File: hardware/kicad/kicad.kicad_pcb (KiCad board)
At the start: 2 copper layers, 4 parts, among them U1 RP2040

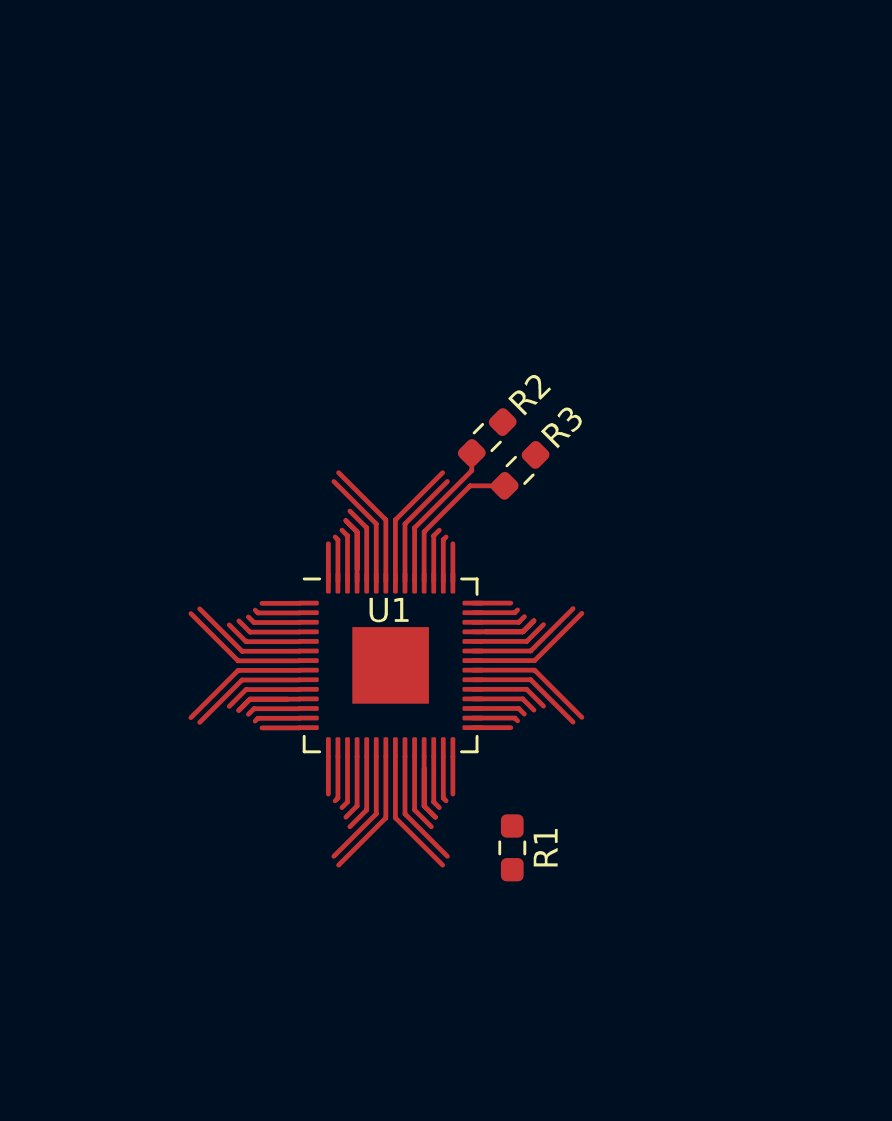
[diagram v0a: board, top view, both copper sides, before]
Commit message: [30-8] update progress
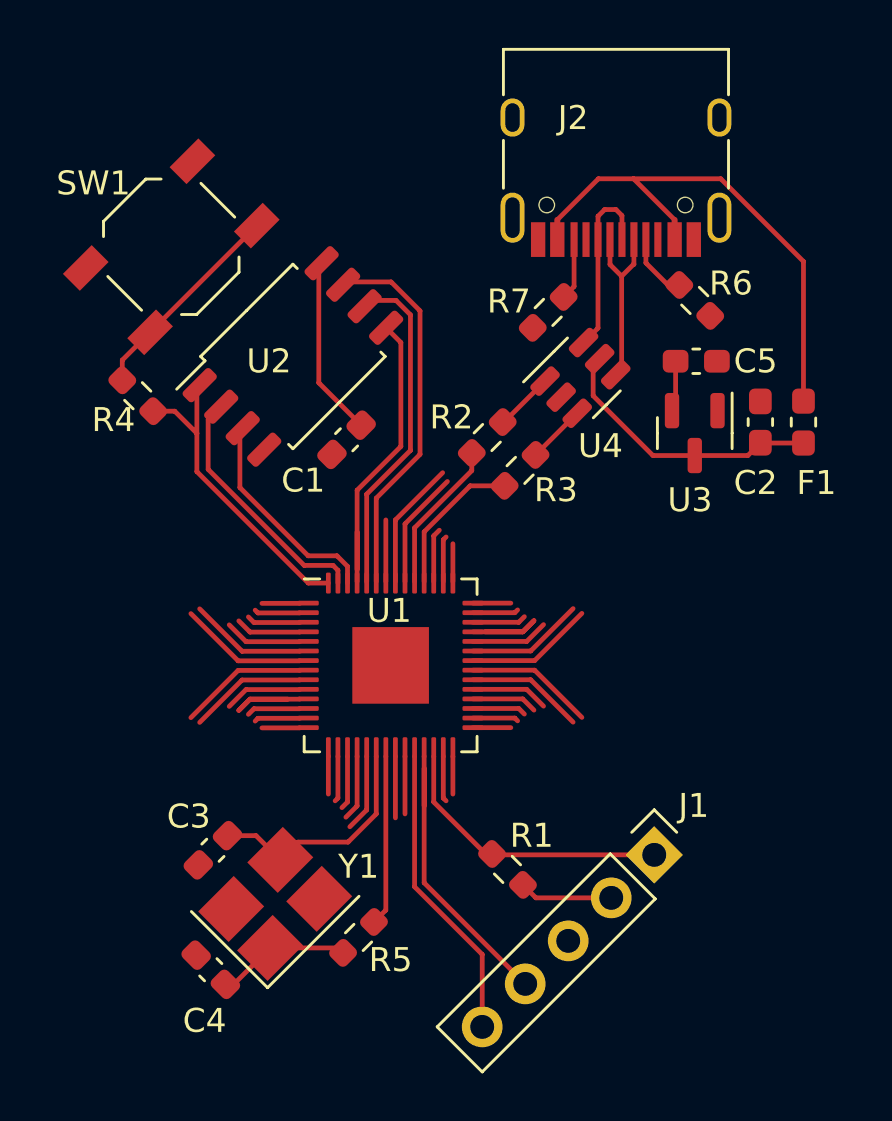
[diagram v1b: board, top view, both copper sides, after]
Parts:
- added C1: C, Capacitor_SMD:C_0603_1608Metric_Pad1.08x0.95mm_HandSolder, F.Cu at (181.0, 74.4)
- added C2: C, Capacitor_SMD:C_0603_1608Metric_Pad1.08x0.95mm_HandSolder, F.Cu at (198.3, 73.7)
- added C3: C, Capacitor_SMD:C_0603_1608Metric_Pad1.08x0.95mm_HandSolder, F.Cu at (175.5, 91.5)
- added C4: C, Capacitor_SMD:C_0603_1608Metric_Pad1.08x0.95mm_HandSolder, F.Cu at (175.4, 96.5)
- added C5: C, Capacitor_SMD:C_0603_1608Metric_Pad1.08x0.95mm_HandSolder, F.Cu at (195.6, 71.1)
- added F1: Polyfuse, Fuse:Fuse_0603_1608Metric_Pad1.05x0.95mm_HandSolder, F.Cu at (200.1, 73.7)
- added J1: Conn_01x05, Connector_PinHeader_2.54mm:PinHeader_1x05_P2.54mm_Vertical, F.Cu at (193.9, 91.7)
- added J2: USB_C_Receptacle_USB2.0, Connector_USB:USB_C_Receptacle_HRO_TYPE-C-31-M-12, F.Cu at (192.3, 62.0)
- added R4: R, Resistor_SMD:R_0603_1608Metric_Pad0.98x0.95mm_HandSolder, F.Cu at (172.3, 72.6)
- added R5: R, Resistor_SMD:R_0603_1608Metric_Pad0.98x0.95mm_HandSolder, F.Cu at (181.5, 95.2)
- added R6: R, Resistor_SMD:R_0603_1608Metric_Pad0.98x0.95mm_HandSolder, F.Cu at (195.6, 68.6)
- added R7: R, Resistor_SMD:R_0603_1608Metric_Pad0.98x0.95mm_HandSolder, F.Cu at (189.5, 69.1)
- added SW1: SW_Push, Button_Switch_SMD:SW_SPST_TL3342, F.Cu at (173.7, 66.3)
- added U2: W25Q128JVS, Package_SO:SOIC-8_5.23x5.23mm_P1.27mm, F.Cu at (178.8, 70.9)
- added U3: XC6206PxxxMR, Package_TO_SOT_SMD:SOT-23, F.Cu at (195.6, 74.1)
- added U4: USBLC6-2SC6, Package_TO_SOT_SMD:SOT-23-6, F.Cu at (190.8, 71.8)
- added Y1: Crystal_GND24_Small, Crystal:Crystal_SMD_3225-4Pin_3.2x2.5mm_HandSoldering, F.Cu at (178.1, 93.8)
- moved R1 0.92 mm to (187.8, 92.3), turned to -45 degrees
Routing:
- net VBUS: track 0.00 -> 22.3 mm
- net CS: track 1.58 -> 13.3 mm
- net +5V: track 0.00 -> 11.7 mm
- net QSPI_CLK: track 3.24 -> 14.2 mm
- net SD3: track 4.92 -> 15.8 mm
- net +3V3: track 28.8 -> 39.6 mm
- net RESET: track 2.25 -> 12.0 mm
- net SWCLK: track 3.24 -> 12.5 mm
- net Net-(R4-Pad2): track 0.00 -> 8.78 mm
- net SD1: track 1.91 -> 10.5 mm
- net SD0: track 4.98 -> 13.2 mm
- net SWD: track 4.98 -> 12.8 mm
- net D_USB_P: track 0.00 -> 7.75 mm
- net D_USB_N: track 0.00 -> 7.70 mm
- net SD2: track 2.25 -> 9.08 mm
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
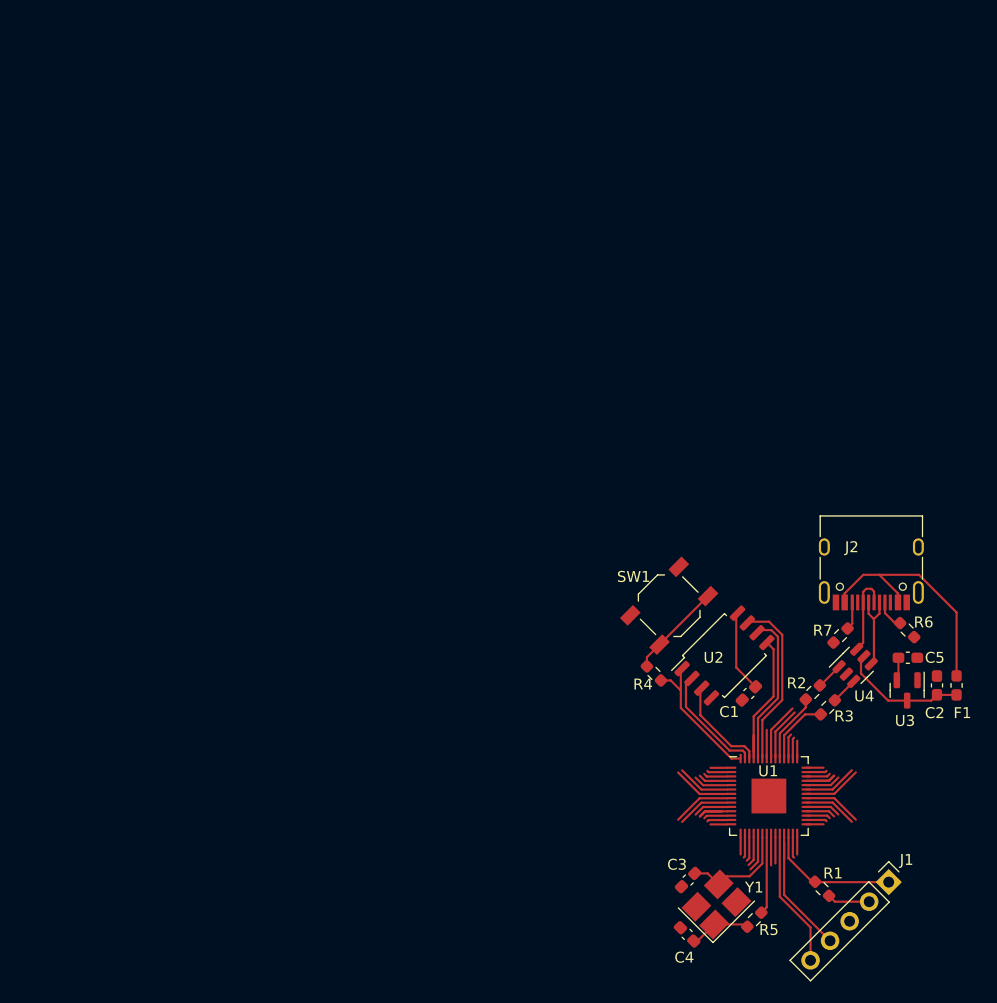
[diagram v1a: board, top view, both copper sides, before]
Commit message: [1-9] update progress
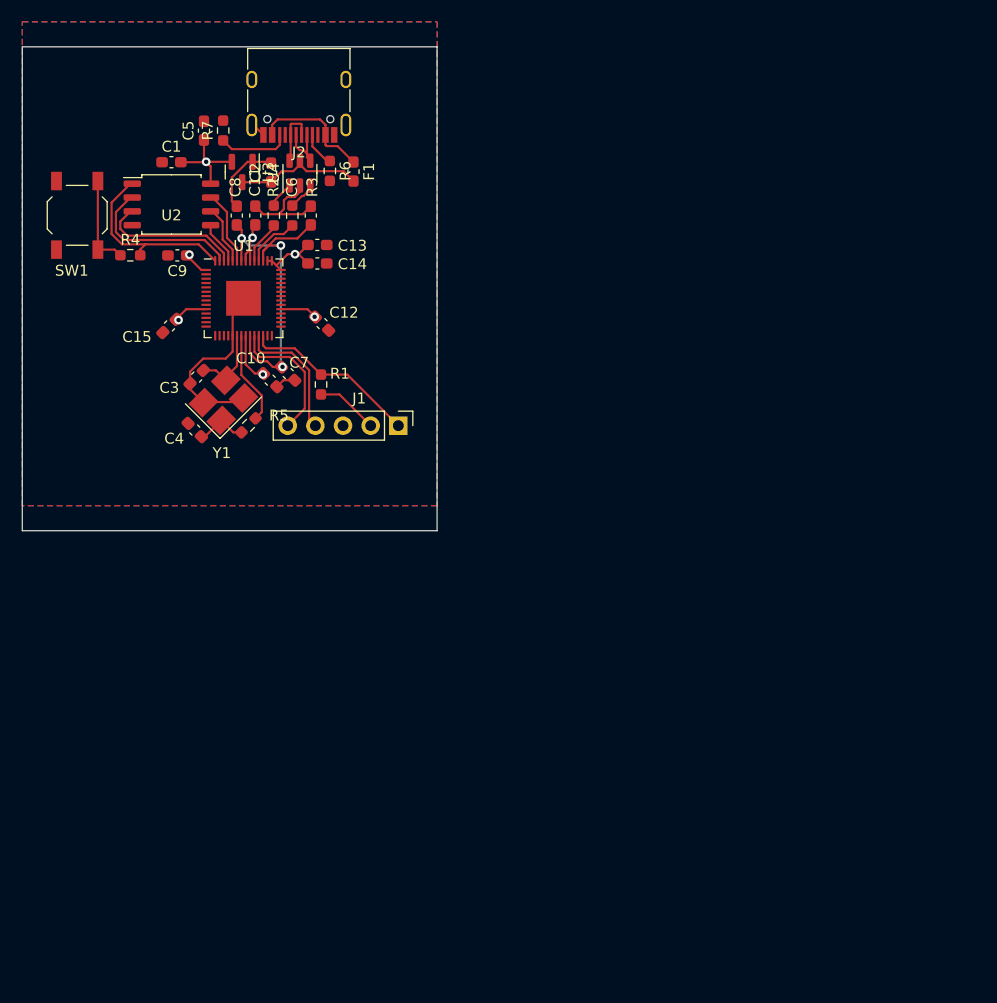
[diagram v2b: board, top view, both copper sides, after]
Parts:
- added C10: C, Capacitor_SMD:C_0603_1608Metric_Pad1.08x0.95mm_HandSolder, F.Cu at (137.1, 45.6)
- added C11: C, Capacitor_SMD:C_0603_1608Metric_Pad1.08x0.95mm_HandSolder, F.Cu at (135.7, 30.5)
- added C12: C, Capacitor_SMD:C_0603_1608Metric_Pad1.08x0.95mm_HandSolder, F.Cu at (141.8, 40.4)
- added C13: C, Capacitor_SMD:C_0603_1608Metric_Pad1.08x0.95mm_HandSolder, F.Cu at (141.4, 33.2)
- added C14: C, Capacitor_SMD:C_0603_1608Metric_Pad1.08x0.95mm_HandSolder, F.Cu at (141.4, 34.9)
- added C15: C, Capacitor_SMD:C_0603_1608Metric_Pad1.08x0.95mm_HandSolder, F.Cu at (127.8, 40.6)
- added C6: C, Capacitor_SMD:C_0603_1608Metric_Pad1.08x0.95mm_HandSolder, F.Cu at (140.8, 30.5)
- added C7: C, Capacitor_SMD:C_0603_1608Metric_Pad1.08x0.95mm_HandSolder, F.Cu at (138.7, 45.0)
- added C8: C, Capacitor_SMD:C_0603_1608Metric_Pad1.08x0.95mm_HandSolder, F.Cu at (134.0, 30.5)
- added C9: C, Capacitor_SMD:C_0603_1608Metric_Pad1.08x0.95mm_HandSolder, F.Cu at (128.5, 34.2)
- moved C5 80.8 mm to (131.0, 22.7), turned to 90 degrees
- moved U3 77.4 mm to (134.5, 26.5)
- moved C2 77.2 mm to (137.2, 26.6)
- moved R7 73.3 mm to (132.8, 22.7), turned to 90 degrees
- moved F1 72.8 mm to (144.7, 26.5)
- moved C1 72.1 mm to (128.0, 25.6), turned to 0 degrees
- moved U4 68.2 mm to (139.8, 26.6), turned to 90 degrees
- moved J2 67.9 mm to (139.7, 19.1)
- moved R6 67.8 mm to (142.6, 26.4), turned to -90 degrees
- moved R3 66.8 mm to (139.1, 30.5), turned to -90 degrees
- moved U1 66.5 mm to (134.6, 38.1)
- moved R2 66.1 mm to (137.4, 30.5), turned to -90 degrees
- moved U2 65.6 mm to (128.0, 29.5), turned to 0 degrees
- moved R1 65.3 mm to (141.7, 46.0), turned to -90 degrees
- moved SW1 65.1 mm to (119.3, 30.5), turned to 90 degrees
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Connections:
- R4 pad 1: CS -> Net-(R4-Pad1)
- R4 pad 2: Net-(R4-Pad2) -> CS
- SW1 pad 2: Net-(R4-Pad2) -> Net-(R4-Pad1)
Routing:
- net GND: track 3.27 -> 34.3 mm
- net +1V1: track 7.23 -> 32.0 mm, vias 0 -> 3
- net VBUS: track 22.3 -> 11.3 mm
- net SD0: track 13.2 -> 3.95 mm
- net SD3: track 15.8 -> 6.75 mm
- net QSPI_CLK: track 14.2 -> 5.32 mm
- net Net-(R4-Pad2): track 8.78 -> 0.00 mm
- net Net-(R4-Pad1): track 0.00 -> 8.58 mm
- net unconnected-(U1-Pad36): track 5.37 -> 0.00 mm
- net unconnected-(U1-Pad8): track 5.37 -> 0.00 mm
- net unconnected-(U1-Pad35): track 5.37 -> 0.00 mm
- net unconnected-(U1-Pad7): track 5.37 -> 0.00 mm
- net unconnected-(U1-Pad39): track 4.98 -> 0.00 mm
- net unconnected-(U1-Pad11): track 4.98 -> 0.00 mm
- net unconnected-(U1-Pad37): track 4.92 -> 0.00 mm
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- added copper zone on B.Cu, net +3V3
- added copper zone on F.Cu, net GND
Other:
- board outline added: 38.1 x 44.5 mm
